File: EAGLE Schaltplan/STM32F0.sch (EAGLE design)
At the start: 8 parts, among them T1 2N1613, X2 MINI-USB_SHIELD5P2-32005-601

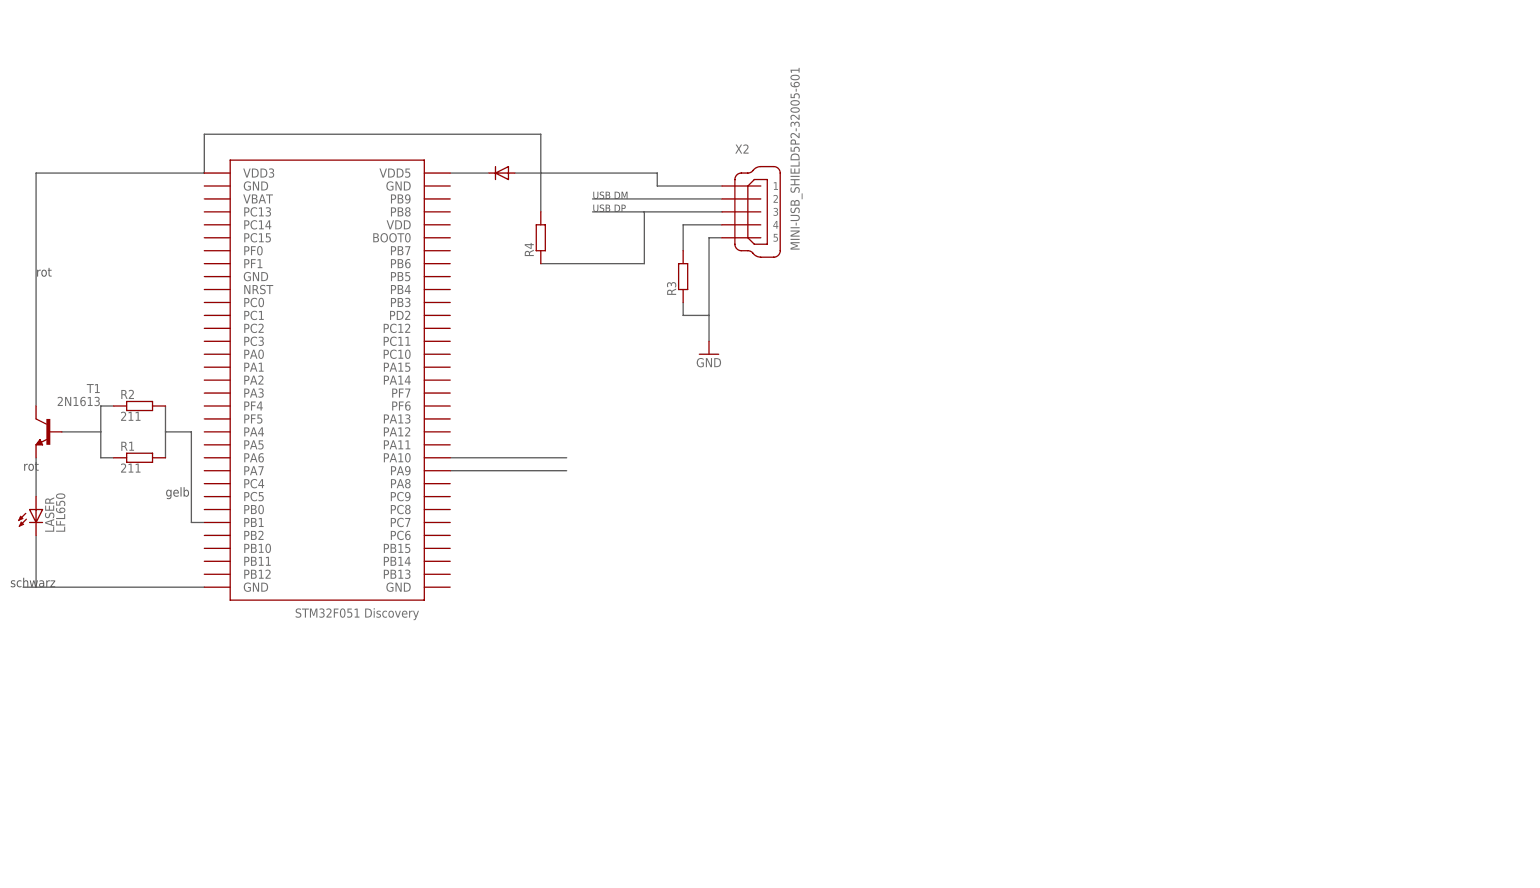
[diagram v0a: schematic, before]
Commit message: EagleFinal
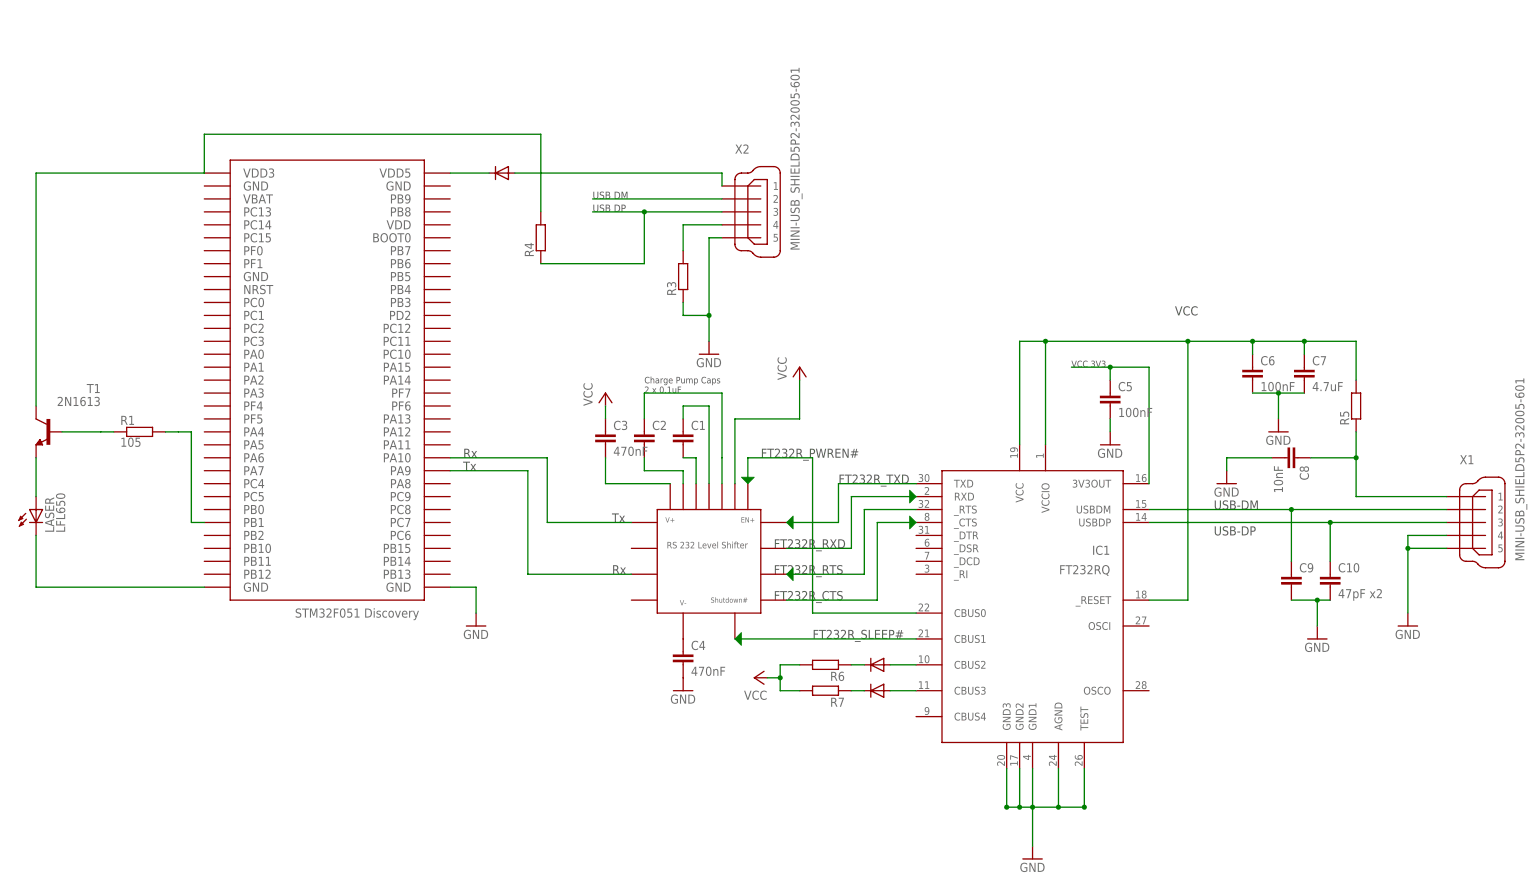
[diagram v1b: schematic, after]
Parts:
- removed R2: 211, resistor-shunt:SMK
- added C1, C2, C9: (no value), capacitor-wima:C22/10
- added C10: 47pF x2, capacitor-wima:C22/10
- added C3, C4: 470nF, capacitor-wima:C22/10
- added C5, C6: 100nF, capacitor-wima:C22/10
- added C7: 4.7uF, capacitor-wima:C22/10
- added C8: 10nF, capacitor-wima:C22/10
- added IC1: FT232RQ, ftdichip-3:FT232RQ
- added R5, R6, R7: (no value), resistor-shunt:SMK
- added U$2: RS232LEVELSHIFTER, RS232 Level Shifter:RS232LEVELSHIFTER
- added X1: MINI-USB_SHIELD5P2-32005-601, con-cypressindustries:MINI-USB_SHIELD5P2-32005-601
- R1: value 211 -> 105
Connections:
- new net GND: C4.2, C5.2, C8.2, R3.2, X2G41.5
- new net N$1: C3.2
- new net N$11: IC1._CTS
- new net N$12: IC1.CBUS0
- new net N$13: IC1.CBUS1
- new net N$14: IC1.AGND, IC1.GND1, IC1.GND2, IC1.GND3, IC1.TEST
- new net N$15: C6.1, C7.1, IC1.VCC, IC1.VCCIO, IC1._RESET, R5.1
- new net N$17: LASER.C
- new net N$18: LASER.A, T1.E
- new net N$19: R4.1, T1.C
- new net N$2: IC1.RXD
- new net N$20: T1.B
- new net N$21: R3.1, X2G41.4
- new net N$22: X2G41.2
- new net N$23: R4.2, X2G41.3
- new net N$25: X2G41.1
- new net N$26: C5.1, IC1.3V3OUT
- new net N$27: C6.2, C7.2
- new net N$28: C8.1, R5.2, X1G41.1
- new net N$29: C9.1, IC1.USBDM, X1G41.2
- new net N$3: C2.1
- new net N$30: C10.1, IC1.USBDP, X1G41.3
- new net N$31: C10.2, C9.2
- new net N$32: X1G41.4, X1G41.5
- new net N$35: IC1.CBUS2
- new net N$36: IC1.CBUS3
- new net N$37: R6.2
- new net N$38: R7.2
- new net N$39: R6.1, R7.1
- new net N$40: R1.1
- new net N$41: R1.2
- new net N$5: C2.2
- new net N$6: IC1.TXD
- new net N$7: IC1._RTS
- new net N$8: C1.2
- new net N$9: C1.1
- new net VCC: C3.1
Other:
- note added: "Charge Pump Caps 2 x 0.1uF"
- note added: "FT232R_CTS"
- note added: "FT232R_PWREN#"
- note added: "FT232R_RTS"
- note added: "FT232R_RXD"
- note added: "FT232R_SLEEP#"
- note added: "FT232R_TXD"
- note added: "Rx"
- note added: "Tx"
- note added: "USB-DM"
- note added: "USB-DP"
- note added: "VCC"
- note added: "VCC 3V3"
- note removed: "gelb"
- note removed: "rot"
- note removed: "schwarz"
- moved on the sheet: R1
